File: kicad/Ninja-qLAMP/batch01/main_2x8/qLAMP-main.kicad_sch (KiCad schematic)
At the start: 16 parts, among them Q3 Q_NMOS_GSD, Q5 Q_NMOS_GSD, U5 ESP32-WROOM-32, U6 ESP32-WROOM-32U

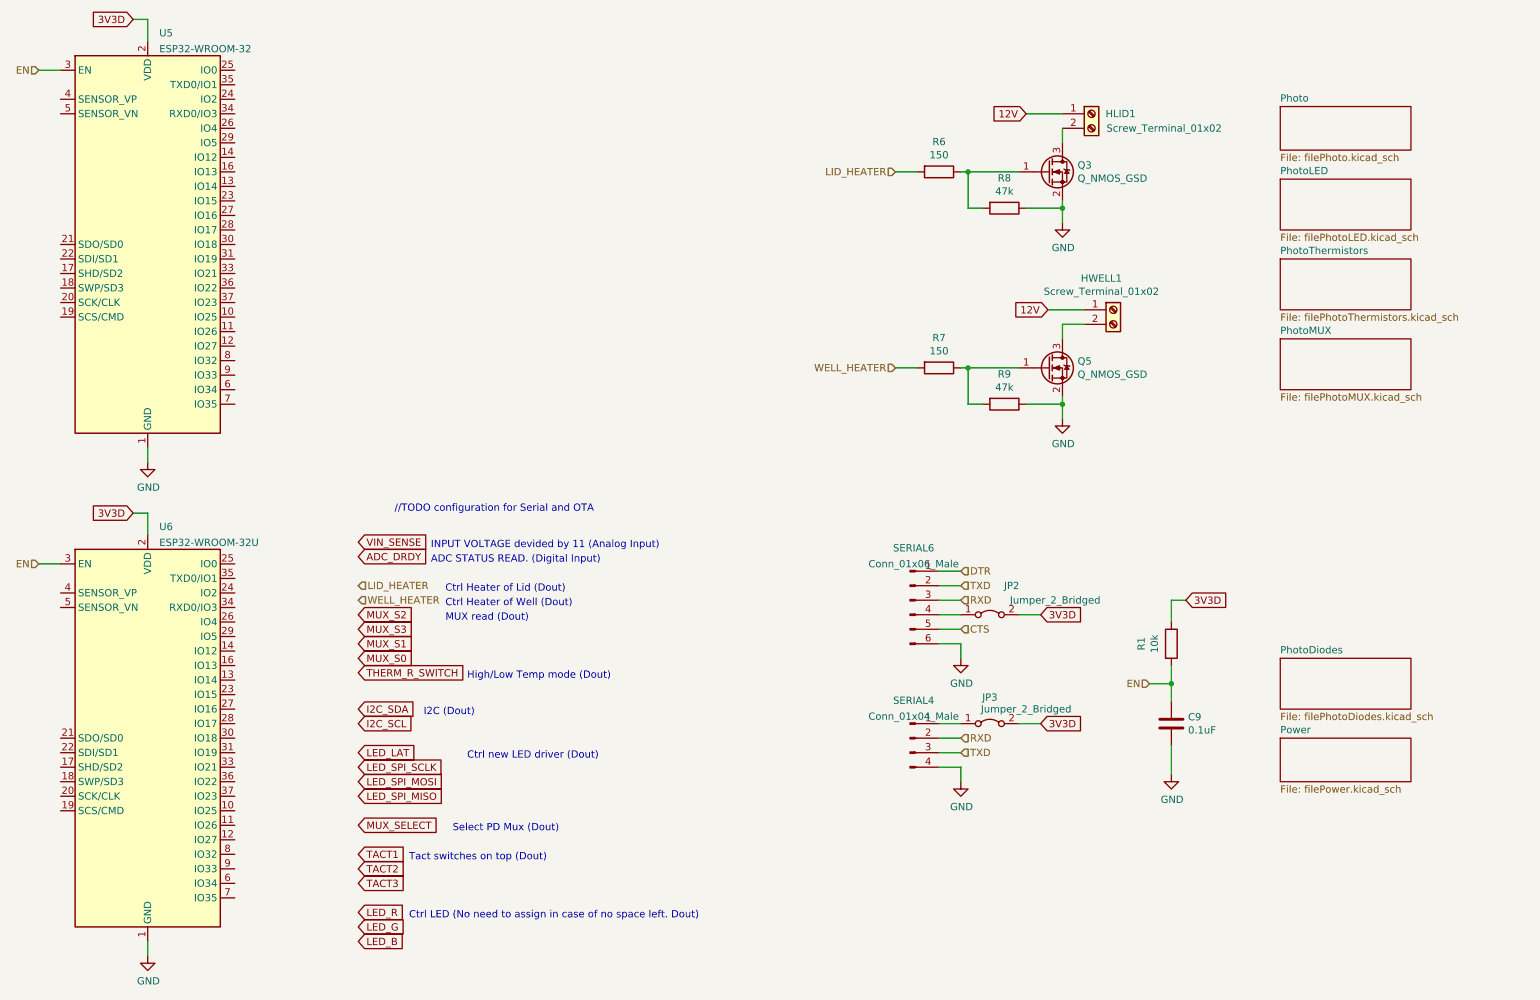
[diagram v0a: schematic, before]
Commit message: sync
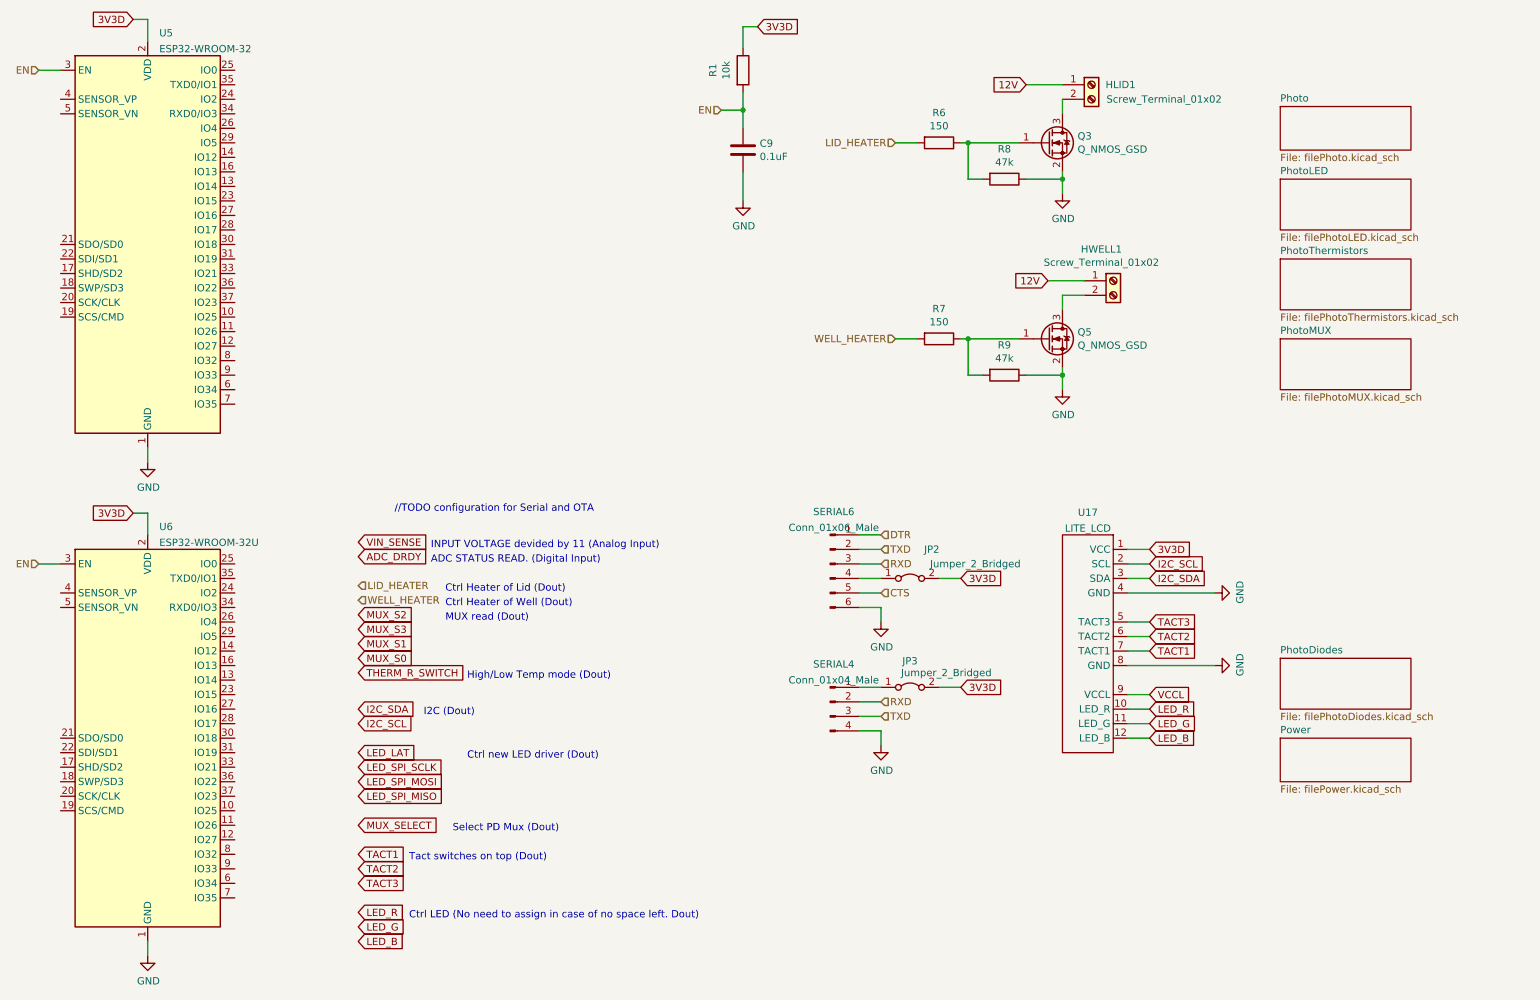
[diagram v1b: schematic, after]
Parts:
- added U17: LITE_LCD, Ninja-qPCR:LITE_LCD, symbol Ninja-qPCR:LITE_LCD
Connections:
- net 3V3D: now also U17.1 (VCC)
- net GND: now also U17.4 (GND), U17.8 (GND)
- net I2C_SCL: now also U17.2 (SCL)
- net I2C_SDA: now also U17.3 (SDA)
- net LED_B: now also U17.12 (LED_B)
- net LED_G: now also U17.11 (LED_G)
- net LED_R: now also U17.10 (LED_R)
- net TACT1: now also U17.7 (TACT1)
- net TACT2: now also U17.6 (TACT2)
- net TACT3: now also U17.5 (TACT3)
- new net VCCL: U17.9 (VCCL)
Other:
- moved on the sheet: C9, HLID1, HWELL1, JP2, JP3, Q3, Q5, R1, R6, R7, R8, R9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
